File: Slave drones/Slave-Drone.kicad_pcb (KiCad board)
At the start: 4 copper layers, 32 x 32 mm, 46 parts, among them J1 Conn_01x02, J2 Conn_01x02, J3 Conn_01x02, J4 Conn_01x02, J5 USB_C_Receptacle_USB2.0_16P, J6 Conn_01x02, SW1 SW_Push, SW2 SW_Push, U1 MPU6500, U2 QMC5883L, U3 ESP32-S3-MINI-1, U4 AP2112K-3.3

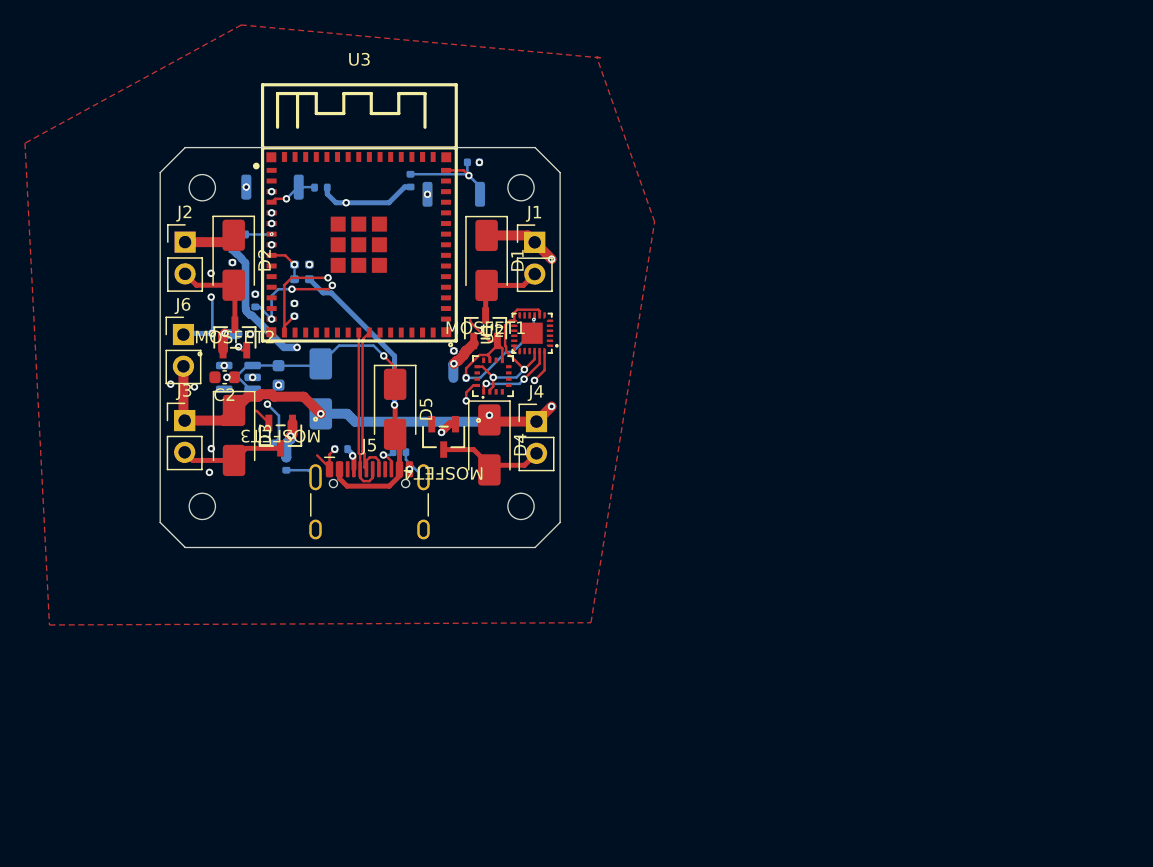
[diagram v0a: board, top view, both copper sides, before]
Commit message: I broke the pcb file, had to restart routing
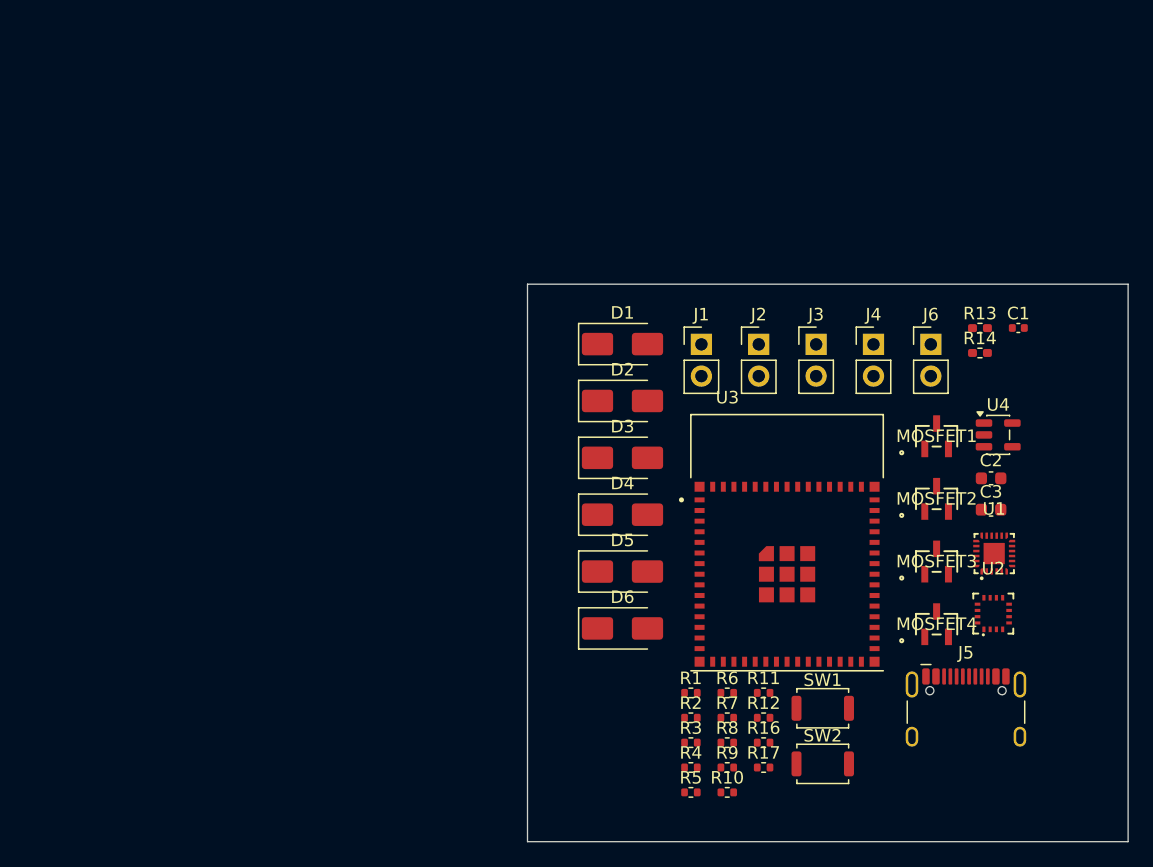
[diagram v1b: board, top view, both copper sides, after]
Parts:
- removed G***: LOGO, LOGO
- removed REF** (x4): MountingHole_2.1mm, MountingHole:MountingHole_2.1mm
- C1, C3, D6, R1, R10, R11, R12, R13, R14, R16, R17, R2, R3, R4, R5, R6, R7, R8, R9, SW1, SW2, U4: moved to F.Cu
- U3: footprint footprint-JLC:BULETM-SMD_ESP32-S3-MINI-1-N8 -> ESP32-S3-MINI-1-N8:XCVR_ESP32-S3-MINI-1-N8
- moved C2 61.9 mm to (164.9, 90.5), turned to 0 degrees
- moved U4 61.0 mm to (165.4, 87.0), turned to 0 degrees
- moved SW1 60.6 mm to (151.4, 108.9), turned to 0 degrees
- moved J6 59.8 mm to (160.1, 79.7)
- moved C3 58.0 mm to (164.9, 93.0), turned to 0 degrees
- moved MOSFET2 57.6 mm to (160.5, 92.1)
- moved R11 55.7 mm to (146.7, 107.6)
- moved R8 55.0 mm to (143.8, 111.6), turned to 0 degrees
- moved R4 55.0 mm to (140.9, 113.6), turned to 0 degrees
- moved R14 54.6 mm to (164.0, 80.4), turned to 0 degrees
- moved R13 54.5 mm to (164.0, 78.4)
- moved SW2 54.3 mm to (151.4, 113.3), turned to 0 degrees
- moved MOSFET3 53.4 mm to (160.5, 97.1), turned to 0 degrees
- moved R5 52.6 mm to (140.9, 115.6), turned to 0 degrees
- moved R9 51.9 mm to (143.8, 113.6)
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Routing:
- net /Motor_Power: track 72.5 -> 0.00 mm, vias 4 -> 0
- net GND: track 42.5 -> 0.00 mm, vias 20 -> 0
- net /SDA: track 33.9 -> 0.00 mm, vias 5 -> 0
- net /SCL: track 32.0 -> 0.00 mm, vias 4 -> 0
- net /Motor3: track 27.7 -> 0.00 mm, vias 2 -> 0
- net Net-(D5-A): track 25.9 -> 0.00 mm, vias 1 -> 0
- net +3.3V: track 24.4 -> 0.00 mm, vias 8 -> 0
- net Net-(U3-IO2): track 18.4 -> 0.00 mm, vias 2 -> 0
- net Net-(U3-IO4): track 18.1 -> 0.00 mm, vias 2 -> 0
- net /USBPWR: track 17.4 -> 0.00 mm, vias 1 -> 0
- net /USB_D+: track 14.0 -> 0.00 mm
- net /USB_D-: track 13.6 -> 0.00 mm
- net Net-(U3-IO1): track 10.7 -> 0.00 mm, vias 2 -> 0
- net /RESET: track 9.70 -> 0.00 mm, vias 1 -> 0
- net Net-(D3-A): track 8.35 -> 0.00 mm
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- removed copper zone on In2.Cu, net +3.3V
- removed copper zone on F.Cu, net GND
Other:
- board size 32 x 32 mm -> 48.1 x 44.6 mm
- copper layers 4 -> 2
